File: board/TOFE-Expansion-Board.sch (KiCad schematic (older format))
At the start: 1 part, among them U1 TOFE-8X

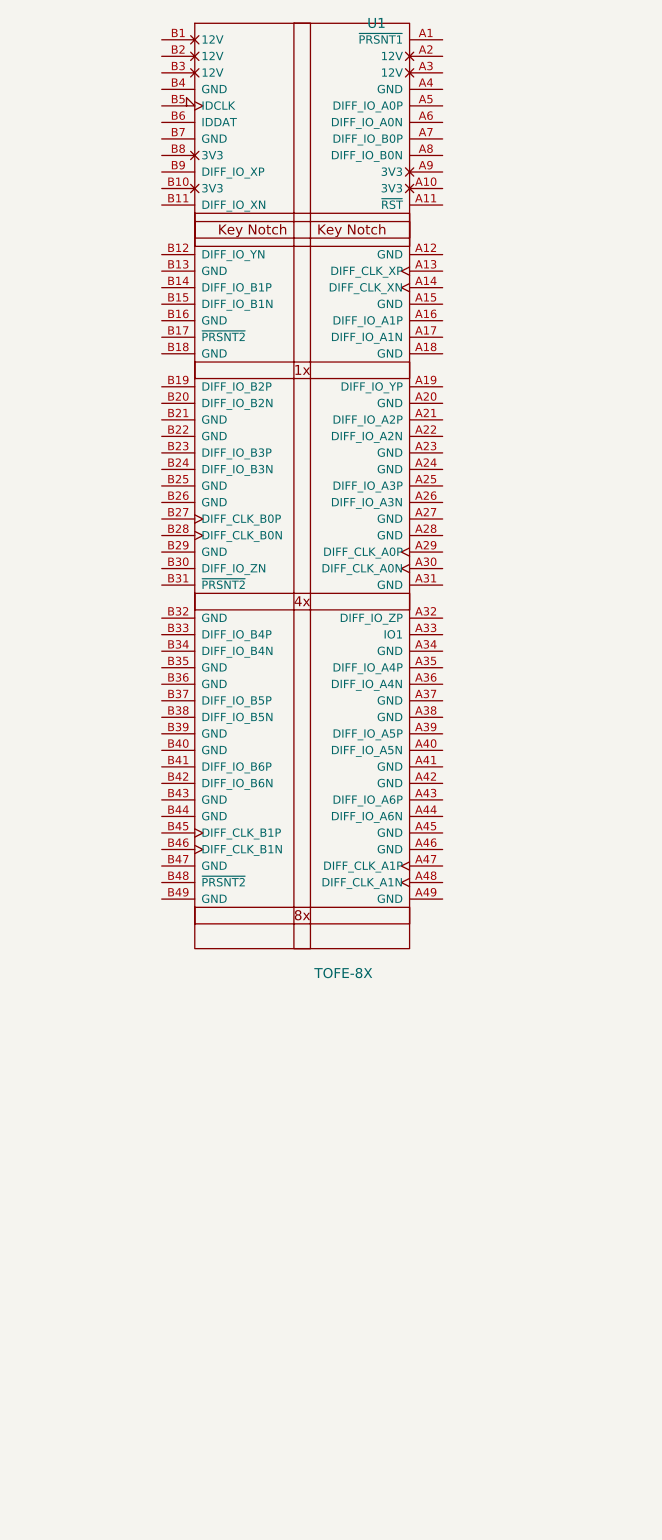
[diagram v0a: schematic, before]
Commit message: Update from Anoop.
Fixes #1.
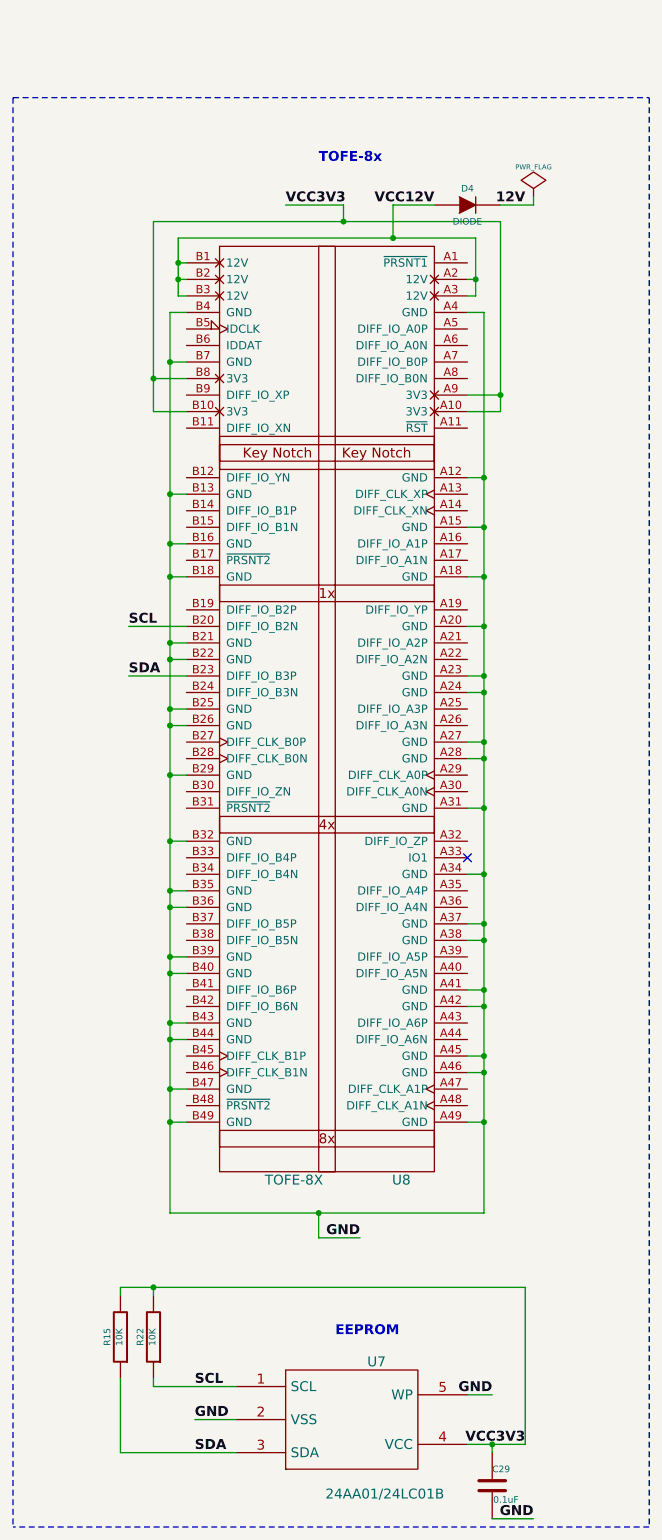
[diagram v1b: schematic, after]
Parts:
- added C29: 0.1uF, ~, symbol C
- added D4: DIODE, ~, symbol DIODE
- added R15, R22: 10K, ~, symbol R
- added U7: 24AA01/24LC01B, ~, symbol 24AA01/24LC01B
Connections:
- net VCC3V3: now reaches U1.A10 (3V3)
- net VCC3V3: now also U1.A9 (3V3), U1.B10 (3V3), U1.B8 (3V3), C29.1, R15.2, R22.2, U7.4 (VCC)
- net GND: now reaches U1.A12 (GND)
- net GND: now also U1.A15 (GND), U1.A18 (GND), U1.A20 (GND), U1.A23 (GND), U1.A24 (GND), U1.A27 (GND), U1.A28 (GND), U1.A31 (GND), U1.A34 (GND), U1.A37 (GND), U1.A38 (GND), U1.A4 (GND), U1.A41 (GND), U1.A42 (GND), U1.A45 (GND), U1.A46 (GND), U1.A49 (GND), U1.B13 (GND), U1.B16 (GND), U1.B18 (GND), U1.B21 (GND), U1.B22 (GND), U1.B25 (GND), U1.B26 (GND), U1.B29 (GND), U1.B32 (GND), U1.B35 (GND), U1.B36 (GND), U1.B39 (GND), U1.B4 (GND), U1.B40 (GND), U1.B43 (GND), U1.B44 (GND), U1.B47 (GND), U1.B49 (GND), U1.B7 (GND), C29.2, U7.2 (VSS), U7.5 (WP)
- net VCC12V: now reaches U1.A2 (12V)
- net VCC12V: now also U1.A3 (12V), U1.B1 (12V), U1.B2 (12V), U1.B3 (12V), D4.1 (A)
- net SCL: now reaches U1.B20 (DIFF_IO_B2N)
- net SCL: now also R22.1, U7.1 (SCL)
- net SDA: now reaches U1.B23 (DIFF_IO_B3P)
- net SDA: now also R15.1, U7.3 (SDA)
- new net 12V: D4.2 (K)
- no-connect marks 0 -> 1
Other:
- note added: "EEPROM"
- note added: "TOFE-8x"
